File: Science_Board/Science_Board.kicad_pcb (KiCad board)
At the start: 2 copper layers, 105.5 x 87 mm, 145 parts, among them IC1 TCKE603RA, IC2 TCKE603RA, IC3 TCKE603RM, J1 Conn_01x02, J10 Conn_01x02, J11 Conn_01x03, J12 Conn_01x03, J13 Conn_01x03, J14 Conn_01x03, J15 Conn_01x03, J16 Conn_01x03, J17 Conn_01x03, J18 Conn_01x03, J19 Conn_01x02, J2 RJ45_LED_Shielded, J20 Molex_Megafit_02, J21 Molex_Megafit_02, J22 Molex_Megafit_02, J23 Conn_01x02, J24 Conn_01x02, J3 Molex_Megafit_02, J4 Molex_Megafit_02, J5 Conn_01x05, J6 Conn_01x04, J7 Conn_01x03, J8 Conn_01x03, J9 Conn_01x02, Q1 BS250, Q2 NMOS, Q3 NMOS, Q4 NMOS, Q5 NMOS, Q6 NMOS, SW1 SW_Push, SW10 SW_Push, SW11 SW_Push, SW12 SW_SPDT, SW2 SW_Push, SW3 SW_Push, SW4 SW_Push, SW5 SW_Push, SW6 SW_Push, SW7 SW_Push, SW8 SW_Push, SW9 SW_Push, U3 LM22678TJ-5, U5 PCA9685PW

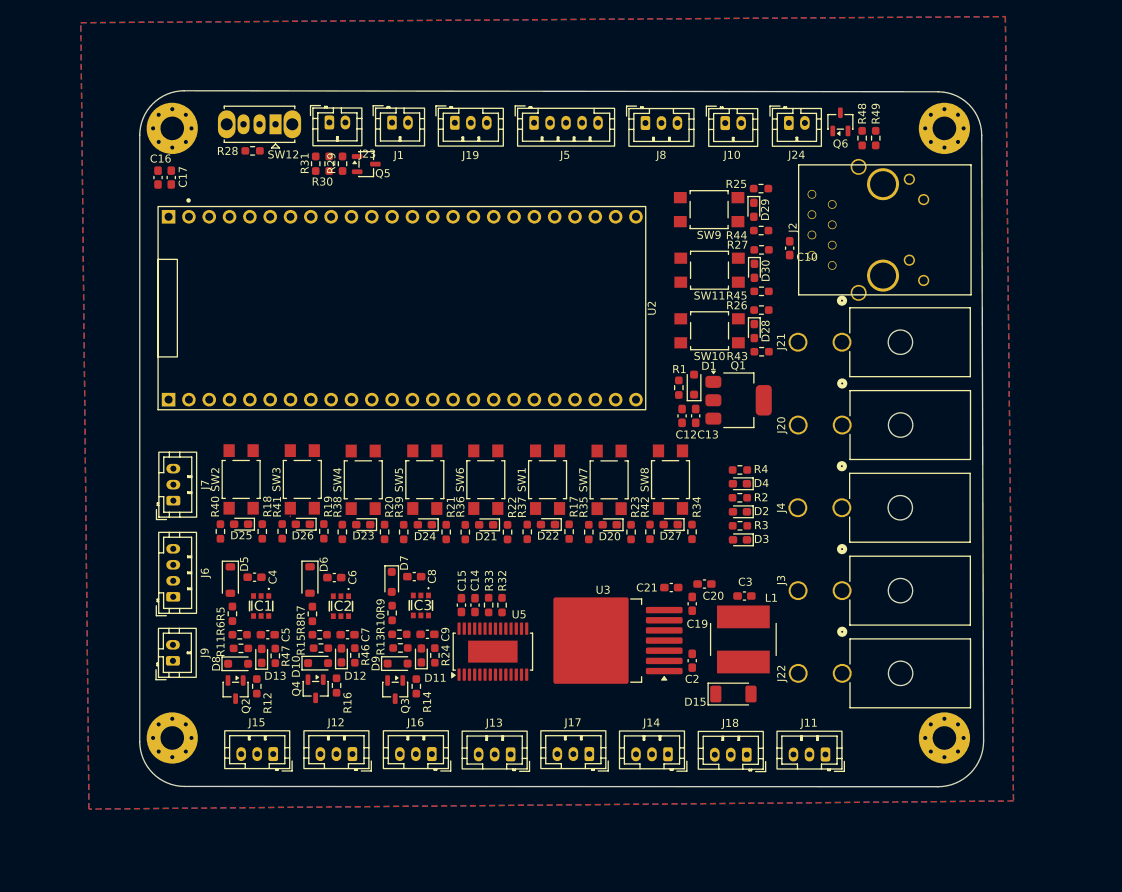
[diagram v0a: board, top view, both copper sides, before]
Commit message: crisp dimensions
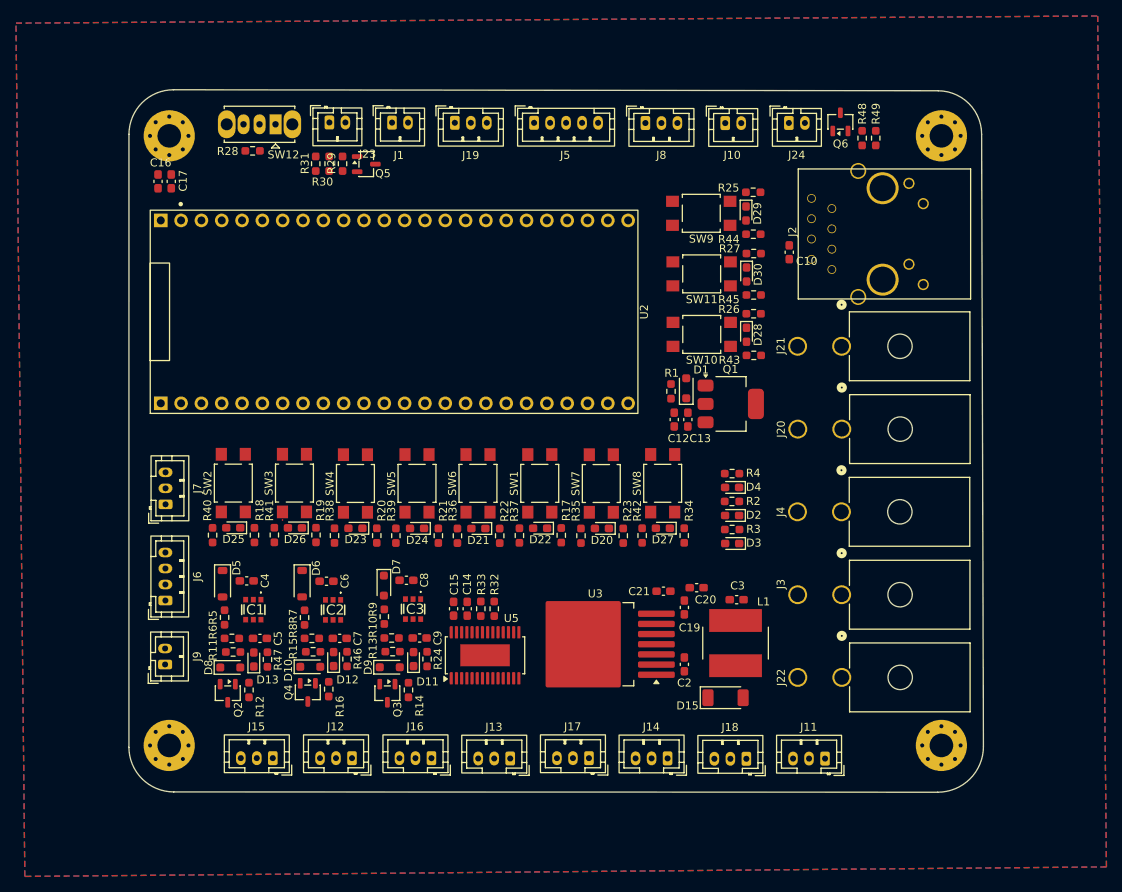
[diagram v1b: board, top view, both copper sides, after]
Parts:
- moved C12 1.08 mm to (149.1, 102.4)
- moved C13 1.08 mm to (150.8, 102.4)
- moved C14 1.08 mm to (123.2, 126.1)
- moved C19 1.08 mm to (150.4, 125.9)
- moved C2 1.08 mm to (150.4, 133.0)
- moved C21 1.08 mm to (147.8, 123.9)
- moved C4 1.08 mm to (95.7, 122.6)
- moved C5 1.08 mm to (97.3, 129.8)
- moved C6 1.08 mm to (105.6, 122.7)
- moved C8 1.08 mm to (115.6, 122.5)
- moved D1 1.08 mm to (150.6, 98.5)
- moved D10 1.08 mm to (103.6, 133.3)
- moved D13 1.08 mm to (96.6, 132.4)
- moved D15 1.08 mm to (155.5, 137.2)
- moved D2 1.08 mm to (156.3, 114.4)
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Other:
- board size 105.5 x 87 mm -> 106.8 x 87.8 mm
